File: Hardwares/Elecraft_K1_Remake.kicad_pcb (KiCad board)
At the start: 2 copper layers, 81.3 x 91.4 mm, 122 parts, among them J1 RF_IN, J10 Conn_01x01, J11 Conn_01x01, J12 Conn_01x01, J13 Conn_01x01, J14 Conn_01x01, J2 PWR_12V, J3 Premix_Filter, J4 Freq_Counter, J5 VFO_Out, J6 Outer_Ctrl, J7 SMTR, J8 Audio, J9 Conn_01x01, Q1 S9018, Q2 2N3904, Q3 2N3906, Q4 2N3904, Q5 2N7000, Q6 2N3906, Q7 MPSA14_EBC, Q8 2N7000, T1 4:20, T2 5:20, U1 L78L05_TO92, U2 SA602, U3 L78L05_TO92, U4 SA602, U5 LM386, U6 SA602, U7 LM380N-8, Y1 4.915MHz, Y2 4.915MHz, Y3 4.915MHz, Y4 4.915MHz, Y5 4.915MHz

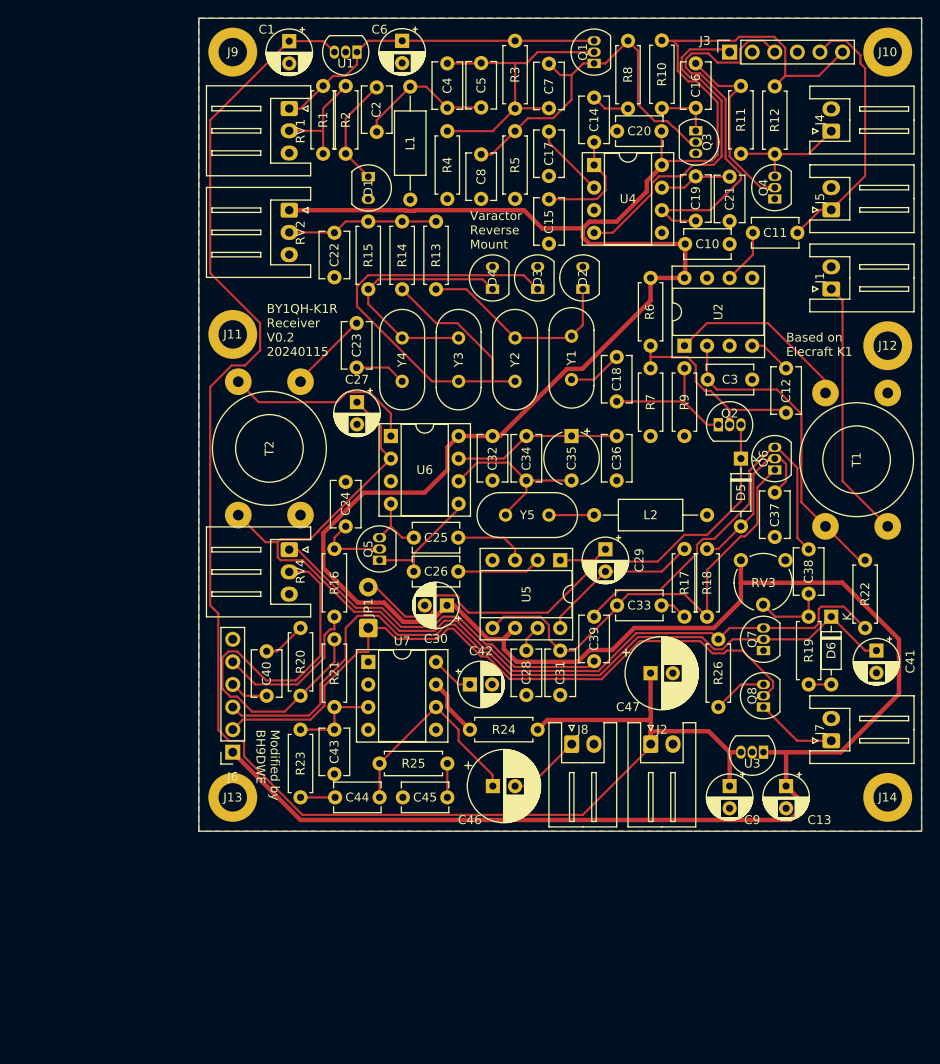
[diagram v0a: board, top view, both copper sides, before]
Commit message: Add files via upload
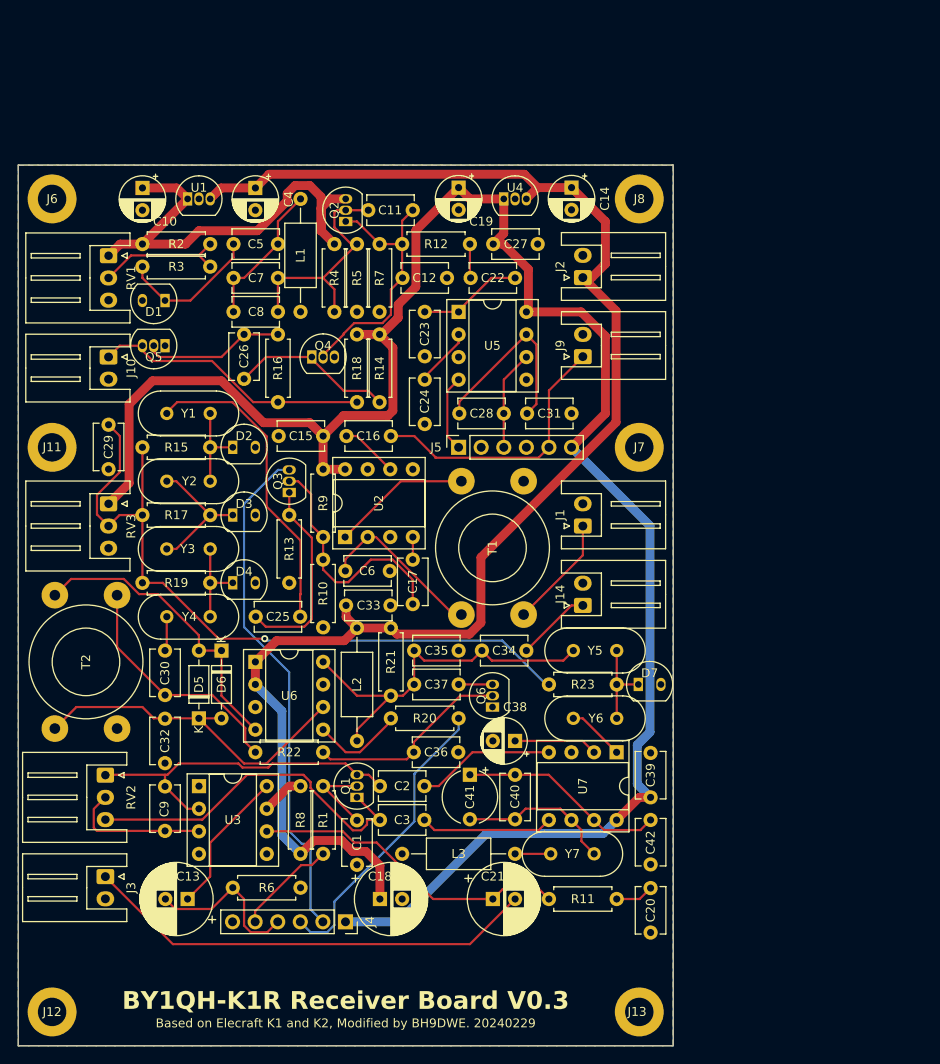
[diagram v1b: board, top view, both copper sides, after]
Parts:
- removed C43: .01u, Capacitor_THT:C_Disc_D5.1mm_W3.2mm_P5.00mm
- removed C44: 220, Capacitor_THT:C_Disc_D5.1mm_W3.2mm_P5.00mm
- removed C45: .047u, Capacitor_THT:C_Disc_D5.1mm_W3.2mm_P5.00mm
- removed C46, C47: 220u, Capacitor_THT:CP_Radial_D8.0mm_P2.50mm
- removed JP1: JMP, Connector_Wire:SolderWire-0.5sqmm_1x02_P4.6mm_D0.9mm_OD2.1mm
- removed Q7: MPSA14_EBC, Package_TO_SOT_THT:TO-92_Inline
- removed Q8: 2N7000, Package_TO_SOT_THT:TO-92_Inline
- removed R24: 10, Resistor_THT:R_Axial_DIN0207_L6.3mm_D2.5mm_P7.62mm_Horizontal
- removed R25: 1.5, Resistor_THT:R_Axial_DIN0207_L6.3mm_D2.5mm_P7.62mm_Horizontal
- removed R26: 27k, Resistor_THT:R_Axial_DIN0207_L6.3mm_D2.5mm_P7.62mm_Horizontal
- removed RV4: 100k, Connector_JST:JST_XH_S3B-XH-A_1x03_P2.50mm_Horizontal
- added D7: ISV149, Package_TO_SOT_THT:TO-92-2, F.Cu at (109.1, 124.5)
- added L3: 47u, Inductor_THT:L_Axial_L7.0mm_D3.3mm_P12.70mm_Horizontal_Fastron_MICC, F.Cu at (95.2, 143.5)
- added Y6: 4.915MHz, Crystal:Crystal_HC49-U_Vertical, F.Cu at (106.7, 128.3)
- added Y7: 4.915MHz, Crystal:Crystal_HC49-U_Vertical, F.Cu at (104.1, 143.5)
- C1: value 10u -> .047u; footprint Capacitor_THT:CP_Radial_D5.0mm_P2.50mm -> Capacitor_THT:C_Disc_D5.1mm_W3.2mm_P5.00mm
- C10: value 0.47u -> 10u; footprint Capacitor_THT:C_Disc_D5.1mm_W3.2mm_P5.00mm -> Capacitor_THT:CP_Radial_D5.0mm_P2.50mm
- C11, C12: value .001u -> 1000
- C13: value 10u -> 22u; footprint Capacitor_THT:CP_Radial_D5.0mm_P2.50mm -> Capacitor_THT:CP_Radial_D8.0mm_P2.50mm
- C14: value .01u -> 10u; footprint Capacitor_THT:C_Disc_D5.1mm_W3.2mm_P5.00mm -> Capacitor_THT:CP_Radial_D5.0mm_P2.50mm
- C15: value 220 -> 0.47u
- C16: value 100 -> 1000
- C17: value .01u -> 1000
- C18: value 220 -> 220u; footprint Capacitor_THT:C_Disc_D5.1mm_W3.2mm_P5.00mm -> Capacitor_THT:CP_Radial_D8.0mm_P2.50mm
- C19: value 39 -> 10u; footprint Capacitor_THT:C_Disc_D5.1mm_W3.2mm_P5.00mm -> Capacitor_THT:CP_Radial_D5.0mm_P2.50mm
- C2: value 220 -> 0.1u
- C20: value 0.47u -> .047u
- C21: value 39 -> 220u; footprint Capacitor_THT:C_Disc_D5.1mm_W3.2mm_P5.00mm -> Capacitor_THT:CP_Radial_D8.0mm_P2.50mm
- C24: value .047u -> .01u
- C25: value 0.1u -> 220
- C26: value 0.1u -> 100
- C27: value 2.2u -> 0.47u; footprint Capacitor_THT:CP_Radial_D5.0mm_P2.50mm -> Capacitor_THT:C_Disc_D5.1mm_W3.2mm_P5.00mm
- C28: value 1u -> 39
- C29, C6, C9: value 10u -> .01u; footprint Capacitor_THT:CP_Radial_D5.0mm_P2.50mm -> Capacitor_THT:C_Disc_D5.1mm_W3.2mm_P5.00mm
- C3: value .01u -> 0.1u
- C30: value 10u -> 220; footprint Capacitor_THT:CP_Radial_D5.0mm_P2.50mm -> Capacitor_THT:C_Disc_D5.1mm_W3.2mm_P5.00mm
- C31: value .01u -> 39
- C32: value 0.47u -> .01u
- C33: value .01u -> 0.47u
- C34: value 22 -> .01u
- C35: value 50 -> 180; footprint Capacitor_THT:CP_Radial_Tantal_D6.0mm_P5.00mm -> Capacitor_THT:C_Disc_D5.1mm_W3.2mm_P5.00mm
- C36: value 330 -> .01u
- C37: value .01u -> 100
- C38: value .1u -> 2.2u; footprint Capacitor_THT:C_Disc_D5.1mm_W3.2mm_P5.00mm -> Capacitor_THT:CP_Radial_D5.0mm_P2.50mm
- C39: value .1u -> 0.47u
- C4: value 220 -> 10u; footprint Capacitor_THT:C_Disc_D5.1mm_W3.2mm_P5.00mm -> Capacitor_THT:CP_Radial_D5.0mm_P2.50mm
- C40: value .01u -> 22
- C41: value 2.2u -> 50; footprint Capacitor_THT:CP_Radial_D5.0mm_P2.50mm -> Capacitor_THT:CP_Radial_Tantal_D6.0mm_P5.00mm
- C42: value 10u -> 330; footprint Capacitor_THT:CP_Radial_D5.0mm_P2.50mm -> Capacitor_THT:C_Disc_D5.1mm_W3.2mm_P5.00mm
- C5, C7: value 1000 -> 220
- D6: value 1N5711 -> 1N4148
- J10: value Conn_01x01 -> Freq_Counter; footprint MountingHole:MountingHole_3.2mm_M3_ISO14580_Pad -> Connector_JST:JST_XH_S2B-XH-A_1x02_P2.50mm_Horizontal
- J14: value Conn_01x01 -> IF_Out; footprint MountingHole:MountingHole_3.2mm_M3_ISO14580_Pad -> Connector_JST:JST_XH_S2B-XH-A_1x02_P2.50mm_Horizontal
- J3: value Premix_Filter -> Audio; footprint Connector_PinSocket_2.54mm:PinSocket_1x06_P2.54mm_Vertical -> Connector_JST:JST_XH_S2B-XH-A_1x02_P2.50mm_Horizontal
- J4: value Freq_Counter -> Outer_Ctrl; footprint Connector_JST:JST_XH_S2B-XH-A_1x02_P2.50mm_Horizontal -> Connector_PinSocket_2.54mm:PinSocket_1x06_P2.54mm_Vertical
- J5: value VFO_Out -> Premix_Filter; footprint Connector_JST:JST_XH_S2B-XH-A_1x02_P2.50mm_Horizontal -> Connector_PinSocket_2.54mm:PinSocket_1x06_P2.54mm_Vertical
- J6: value Outer_Ctrl -> Conn_01x01; footprint Connector_PinSocket_2.54mm:PinSocket_1x06_P2.54mm_Vertical -> MountingHole:MountingHole_3.2mm_M3_ISO14580_Pad
- J7: value SMTR -> Conn_01x01; footprint Connector_JST:JST_XH_S2B-XH-A_1x02_P2.50mm_Horizontal -> MountingHole:MountingHole_3.2mm_M3_ISO14580_Pad
- J8: value Audio -> Conn_01x01; footprint Connector_JST:JST_XH_S2B-XH-A_1x02_P2.50mm_Horizontal -> MountingHole:MountingHole_3.2mm_M3_ISO14580_Pad
- J9: value Conn_01x01 -> PreMix_Out; footprint MountingHole:MountingHole_3.2mm_M3_ISO14580_Pad -> Connector_JST:JST_XH_S2B-XH-A_1x02_P2.50mm_Horizontal
- L1: value 4.4u -> 47u
- L2: value 33u -> 4.7u
- Q1: value S9018 -> 2N7000
- Q2: value 2N3904 -> S9018
- Q3, Q6: value 2N3906 -> 2N3904
- Q4: value 2N3904 -> 2N3906
- Q5: value 2N7000 -> 2N3904
- R1: value 100k -> 47k
- R10: value 2.7k -> 27k
- R11: value 100k -> 1.5
- R13: value 100k -> 27k
- R14: value 100k -> 2.7k
- R16, R19, R23: value 47k -> 100k
- R17: value 2.7k -> 100k
- R18: value 2.2M -> 2.7k
- R20: value 47k -> 5k
- R21: value 47k -> 5.6k
- R22: value 1.8k -> 3.9k
- R3: value 51k -> 100k
- R5: value 2k -> 51k
- R6: value 27k -> 1k
- R7: value 27k -> 2k
- R8: value 2.7k -> 10
- RV3: value 50k -> 100k; footprint Potentiometer_THT:Potentiometer_Piher_PT-6-V_Vertical -> Connector_JST:JST_XH_S3B-XH-A_1x03_P2.50mm_Horizontal
- U3: value L78L05_TO92 -> LM380N-8; footprint Package_TO_SOT_THT:TO-92_Inline -> Package_DIP:DIP-8_W7.62mm_Socket
- U4: value SA602 -> L78L05_TO92; footprint Package_DIP:DIP-8_W7.62mm_Socket -> Package_TO_SOT_THT:TO-92_Inline
- U5: value LM386 -> SA602
- U6: value SA602 -> MC1350
- U7: value LM380N-8 -> SA602
- moved J12 120.2 mm to (43.2, 161.3)
- moved J3 116.3 mm to (49.2, 146.1), turned to -90 degrees
- moved J4 104.4 mm to (76.2, 151.2), turned to -90 degrees
- moved J10 94.1 mm to (49.5, 87.6), turned to -90 degrees
- moved C1 88.0 mm to (77.5, 139.7)
- moved Q1 86.8 mm to (77.5, 137.2)
- moved C21 85.5 mm to (92.8, 148.6), turned to 0 degrees
- moved C20 85.2 mm to (110.5, 147.4), turned to -90 degrees
- moved R11 85.0 mm to (106.7, 148.6), turned to 180 degrees
- moved R8 84.6 mm to (71.1, 135.9), turned to -90 degrees
- moved R1 78.7 mm to (73.7, 135.9)
- moved R6 77.0 mm to (63.5, 147.3), turned to 0 degrees
- moved R10 76.2 mm to (73.7, 118.0), turned to 90 degrees
- moved C2 73.8 mm to (85.0, 135.9), turned to 180 degrees
- moved R22 71.9 mm to (66.0, 132.1), turned to 0 degrees
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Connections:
- C1 pad 1: +12V -> Net-(Q1-G)
- C10 pad 1: GND -> +5VA
- C10 pad 2: +5V -> GND
- C11 pad 1: Net-(U2-OSC_B) -> Net-(Q2-B)
- C11 pad 2: PreMix -> VFO_Out
- C12 pad 1: Net-(U2-OUT_A) -> VFO_Out
- C12 pad 2: Net-(Q2-B) -> GND
- C13 pad 1: +5V -> Net-(U3-BYPASS)
- C13 pad 2: GND -> SideTone
- C14 pad 1: Net-(U4-IN_A) -> +12V
- C14 pad 2: Net-(C14-Pad2) -> GND
- C15 pad 2: Net-(U4-IN_A) -> +5V
- C16 pad 1: Net-(Q4-B) -> Net-(U2-OSC_B)
- C16 pad 2: Net-(Q3-E) -> PreMix
- C17 pad 1: Net-(U4-IN_B) -> Net-(U2-OUT_A)
- C17 pad 2: GND -> Net-(Q3-B)
- C18 pad 1: Net-(Q2-E) -> +12V
- C18 pad 2: Net-(C18-Pad2) -> GND
- C19 pad 1: Net-(U4-OSC_E) -> +5V
- C19 pad 2: Net-(J3-Pin_3) -> GND
- C2 pad 1: Net-(C2-Pad1) -> AF_1
- C2 pad 2: Net-(D1-K) -> Net-(Q1-D)
- C20 pad 1: GND -> Net-(C20-Pad1)
- C20 pad 2: +5V -> GND
- C21 pad 1: Net-(U4-OSC_E) -> Net-(C21-Pad1)
- C21 pad 2: GND -> Net-(J3-Pin_1)
- C22 pad 1: Net-(C22-Pad1) -> Net-(U5-IN_A)
- C22 pad 2: GND -> Net-(C22-Pad2)
- C23 pad 1: Net-(C23-Pad1) -> GND
- C23 pad 2: Net-(T2-AB) -> Net-(U5-IN_A)
- C24 pad 1: Net-(Q5-G) -> Net-(U5-IN_B)
- C25 pad 1: AF_1 -> Net-(Q3-E)
- C25 pad 2: Net-(U5-+) -> Net-(C25-Pad2)
- C26 pad 1: AF_2 -> Net-(Q5-B)
- C26 pad 2: Net-(U5--) -> Net-(Q4-E)
- C27 pad 1: Coil_2 -> GND
- C27 pad 2: GND -> +5V
- C28 pad 1: Net-(U5-BYPASS) -> Net-(U5-OSC_E)
- C28 pad 2: GND -> Net-(J5-Pin_3)
- C29 pad 1: Net-(C29-Pad1) -> BW_Ctrl
- C29 pad 2: Net-(C29-Pad2) -> GND
- C3 pad 1: Coil_1 -> AF_2
- C3 pad 2: GND -> Net-(Q1-S)
- C30 pad 1: +5V -> Net-(C30-Pad1)
- C30 pad 2: GND -> Coil_2A
- C31 pad 1: Net-(Q6-E) -> Net-(U5-OSC_E)
- C32 pad 1: GND -> Net-(D5-K)
- C32 pad 2: +5V -> GND
- C33 pad 1: Net-(C33-Pad1) -> GND
- C33 pad 2: Net-(Q6-E) -> +12V
- C34 pad 1: Net-(U6-OSC_E) -> Net-(J14-Pin_1)
- C34 pad 2: Net-(U6-OSC_B) -> Net-(U6-OUTB)
- C35 pad 1: Net-(U6-OSC_E) -> GND
- C35 pad 2: Net-(U6-OSC_B) -> Net-(U6-OUTB)
- C36 pad 1: Net-(U6-OSC_E) -> Net-(Q6-B)
- C37 pad 1: Net-(D5-A) -> Net-(Q6-C)
- C37 pad 2: GND -> Net-(U6-OUTB)
- C38 pad 1: AF_level -> Net-(U7-IN_B)
- C38 pad 2: Net-(C38-Pad2) -> GND
- C39 pad 1: AF_level -> GND
- C39 pad 2: Net-(C39-Pad2) -> +5V
- C4 pad 1: Net-(Q1-B) -> +12V
- C4 pad 2: Net-(C2-Pad1) -> GND
- C40 pad 1: XFIL/TONE -> Net-(U7-OSC_E)
- C40 pad 2: Net-(C40-Pad2) -> Net-(U7-OSC_B)
- C41 pad 1: ~{AGC OFF} -> Net-(U7-OSC_E)
- C41 pad 2: GND -> Net-(U7-OSC_B)
- C42 pad 1: Net-(U7-BYPASS) -> Net-(U7-OSC_E)
- C5 pad 1: Net-(Q1-B) -> Net-(C5-Pad1)
- C5 pad 2: Net-(C2-Pad1) -> Net-(D1-K)
- C6 pad 1: +5VA -> Net-(T1-SA)
- C7 pad 1: Net-(Q1-B) -> Net-(Q2-B)
- C7 pad 2: VFO_Out -> Net-(C5-Pad1)
- C8 pad 1: VFO_Out -> Net-(Q2-B)
- C8 pad 2: GND -> Net-(C5-Pad1)
- C9 pad 1: +12V -> Net-(Q1-D)
- C9 pad 2: GND -> Net-(U3--)
- D5 pad 1: 6R/AUX1 -> Net-(D5-K)
- D6 pad 1: ~{AGC OFF} -> Net-(D5-A)
- D6 pad 2: Net-(D6-A) -> Net-(D5-K)
- J10 pad 1: GND -> Net-(J10-Pin_1)
- J14 pad 1: GND -> Net-(J14-Pin_1)
- J4 pad 1: Net-(J4-Pin_1) -> +5V
- J4 pad 2: GND -> 6R/AUX
- J5 pad 1: PreMix -> Net-(J5-Pin_1)
- J6 pad 1: +5V -> GND
- J7 pad 1: Net-(J7-Pin_1) -> GND
- J8 pad 1: Net-(J8-Pin_1) -> GND
- J9 pad 1: GND -> PreMix
- L1 pad 1: Net-(C2-Pad1) -> Net-(C5-Pad1)
- L2 pad 1: Net-(L2-Pad1) -> Net-(U6-OUTB)
- L2 pad 2: GND -> +12V
- Q1 pad 1: VFO_Out -> Net-(Q1-S)
- Q1 pad 2: Net-(Q1-B) -> Net-(Q1-G)
- Q1 pad 3: +5VA -> Net-(Q1-D)
- Q2 pad 1: Net-(Q2-E) -> VFO_Out
- Q2 pad 3: 6R/AUX1 -> +5VA
- Q3 pad 2: VFO_Out -> Net-(Q3-B)
- Q3 pad 3: GND -> 6R/AUX
- Q4 pad 1: GND -> Net-(Q4-E)
- Q4 pad 2: Net-(Q4-B) -> VFO_Out
- Q4 pad 3: Net-(J4-Pin_1) -> GND
- Q5 pad 1: AF_2 -> GND
- Q5 pad 2: Net-(Q5-G) -> Net-(Q5-B)
- Q5 pad 3: AF_1 -> Net-(J10-Pin_1)
- Q6 pad 1: Net-(Q6-E) -> GND
- Q6 pad 2: Net-(D5-A) -> Net-(Q6-B)
- Q6 pad 3: AF_level -> Net-(Q6-C)
- R1 pad 1: +5VA -> Net-(Q1-G)
- R1 pad 2: Net-(R1-Pad2) -> Mute
- R10 pad 1: +5V -> GND
- R10 pad 2: Net-(Q3-E) -> Net-(Q3-B)
- R11 pad 1: Net-(J4-Pin_1) -> Net-(C20-Pad1)
- R11 pad 2: Net-(Q4-B) -> Net-(C21-Pad1)
- R12 pad 1: +5V -> Net-(C22-Pad2)
- R12 pad 2: Net-(J4-Pin_1) -> VFO_Out
- R13 pad 1: Net-(D2-K) -> GND
- R13 pad 2: Net-(C22-Pad1) -> Net-(Q3-E)
- R14 pad 1: Net-(D3-K) -> +5V
- R14 pad 2: Net-(C22-Pad1) -> Net-(Q4-E)
- R15 pad 1: Net-(D4-K) -> Net-(D2-K)
- R15 pad 2: Net-(C22-Pad1) -> BW_Ctrl
- R16 pad 1: Net-(Q5-G) -> Net-(J10-Pin_1)
- R16 pad 2: Mute -> Net-(Q5-B)
- R17 pad 1: Net-(C29-Pad2) -> Net-(D3-K)
- R17 pad 2: Net-(C33-Pad1) -> BW_Ctrl
- R18 pad 1: Net-(D5-A) -> +5V
- R18 pad 2: Net-(Q6-E) -> Net-(J10-Pin_1)
- R19 pad 1: Net-(C38-Pad2) -> Net-(D4-K)
- R19 pad 2: Net-(D6-A) -> BW_Ctrl
- R2 pad 1: Net-(R1-Pad2) -> +5VA
- R2 pad 2: Net-(D1-K) -> Net-(R2-Pad2)
- R20 pad 1: Net-(R20-Pad1) -> AGC
- R20 pad 2: Net-(C40-Pad2) -> Net-(U6-AGC)
- R21 pad 1: Net-(R20-Pad1) -> +12V
- R21 pad 2: Net-(U7--) -> Net-(U6-OUTB)
- R22 pad 1: Coil_1 -> Coil_2A
- R22 pad 2: Coil_2 -> Net-(Q6-B)
- R23 pad 1: Net-(U7--) -> Net-(D7-K)
- R23 pad 2: Net-(C44-Pad1) -> BW_Ctrl
- R3 pad 1: Net-(Q1-B) -> Net-(R2-Pad2)
- R3 pad 2: +5VA -> Net-(D1-K)
- R4 pad 1: GND -> Net-(Q2-B)
- R4 pad 2: Net-(Q1-B) -> +5VA
- R5 pad 1: VFO_Out -> GND
- R5 pad 2: GND -> Net-(Q2-B)
- R6 pad 1: Net-(Q2-B) -> SideTone
- R6 pad 2: +5V -> GND
- R7 pad 1: GND -> VFO_Out
- R7 pad 2: Net-(Q2-B) -> GND
- R8 pad 1: Net-(C14-Pad2) -> Net-(U3-VS)
- R8 pad 2: VFO_Out -> +12V
- R9 pad 1: GND -> Net-(Q3-B)
- R9 pad 2: Net-(Q2-E) -> +5V
- RV1 pad 2: Net-(R1-Pad2) -> Net-(R2-Pad2)
- RV2 pad 1: +5V -> Net-(Q1-D)
- RV2 pad 2: Net-(C22-Pad1) -> Net-(U3--)
- RV2 pad 3: GND -> Net-(Q1-S)
- RV3 pad 2: Net-(C38-Pad2) -> BW_Ctrl
- T1 pad 3: Coil_1 -> Net-(T1-SA)
- T2 pad 2: Net-(T2-AB) -> Coil_2A
- T2 pad 3: Coil_2 -> Net-(D5-K)
- T2 pad 4: Net-(T2-SB) -> Net-(D5-A)
- U2 pad 2: Coil_1 -> Net-(T1-SA)
- U3 pad 1: +5V -> unconnected-(U3-NC-Pad1)
- U3 pad 2: GND -> Net-(Q1-D)
- U3 pad 3: +12V -> Net-(U3--)
- U4 pad 1: Net-(U4-IN_A) -> +5V
- U4 pad 2: Net-(U4-IN_B) -> GND
- U4 pad 3: GND -> +12V
- U5 pad 1: Net-(C29-Pad1) -> Net-(U5-IN_A)
- U5 pad 2: Net-(U5--) -> Net-(U5-IN_B)
- U5 pad 3: Net-(U5-+) -> GND
- U5 pad 4: GND -> Net-(J5-Pin_1)
- U5 pad 5: Net-(Q6-E) -> unconnected-(U5-OUT_B-Pad5)
- U5 pad 6: +5V -> Net-(J5-Pin_3)
- U5 pad 7: Net-(U5-BYPASS) -> Net-(U5-OSC_E)
- U5 pad 8: Net-(C29-Pad2) -> +5V
- U6 pad 1: Net-(T2-SB) -> +12V
- U6 pad 2: Coil_2 -> +12V
- U6 pad 4: AF_1 -> Net-(D5-A)
- U6 pad 5: AF_2 -> Net-(U6-AGC)
- U6 pad 6: Net-(U6-OSC_B) -> Net-(D5-K)
- U6 pad 7: Net-(U6-OSC_E) -> GND
- U6 pad 8: +5V -> Net-(U6-OUTB)
- U7 pad 1: unconnected-(U7-NC-Pad1) -> Net-(U7-IN_A)
- U7 pad 2: GND -> Net-(U7-IN_B)
- U7 pad 3: Net-(U7--) -> GND
- U7 pad 4: GND -> AF_1
- U7 pad 5: GND -> AF_2
- U7 pad 6: Net-(C44-Pad2) -> Net-(U7-OSC_B)
- U7 pad 7: Net-(U7-VS) -> Net-(U7-OSC_E)
- U7 pad 8: Net-(U7-BYPASS) -> +5V
- Y1 pad 1: Net-(C18-Pad2) -> Net-(C25-Pad2)
- Y4 pad 2: Net-(C23-Pad1) -> Net-(C30-Pad1)
- Y5 pad 1: Net-(U6-OSC_B) -> Net-(U6-OUTB)
- Y5 pad 2: Net-(L2-Pad1) -> Net-(D7-K)
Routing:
- net +5V: track 358.4 -> 214.6 mm
- net Coil_2: track 109.8 -> 0.00 mm
- net ~{AGC OFF}: track 89.9 -> 0.00 mm
- net BW_Ctrl: track 0.00 -> 83.5 mm, vias 0 -> 1
- net 6R/AUX1: track 59.2 -> 0.00 mm
- net Net-(Q6-E): track 50.7 -> 0.00 mm
- net Net-(R20-Pad1): track 48.1 -> 0.00 mm
- net Net-(D3-K): track 61.0 -> 15.5 mm
- net Net-(J3-Pin_3): track 44.4 -> 0.00 mm
- net AF_level: track 43.5 -> 0.00 mm
- net Net-(U6-OUTB): track 0.00 -> 42.6 mm
- net Net-(C39-Pad2): track 41.0 -> 0.00 mm
- net Net-(Q1-S): track 0.00 -> 40.4 mm
- net Net-(Q1-D): track 0.00 -> 39.0 mm
- net Net-(D5-K): track 0.00 -> 39.0 mm
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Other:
- board size 81.3 x 91.4 mm -> 73.7 x 99.1 mm
- board text added: "BY1QH-K1R Receiver Board V0.3"
- board text added: "Based on Elecraft K1 and K2, Modified by BH9DWE. 20240229"
- board text removed: "BY1QH-K1R Receiver V0.2 20240115"
- board text removed: "Based on Elecraft K1"
- board text removed: "Correction: Cut here"
- board text removed: "Modified by BH9DWE"
- board text removed: "Varactor Reverse Mount"
